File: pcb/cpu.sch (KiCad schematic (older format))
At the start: 8 parts, among them J100 Conn_02x05_Odd_Even, U100 LPC5500_FBD64

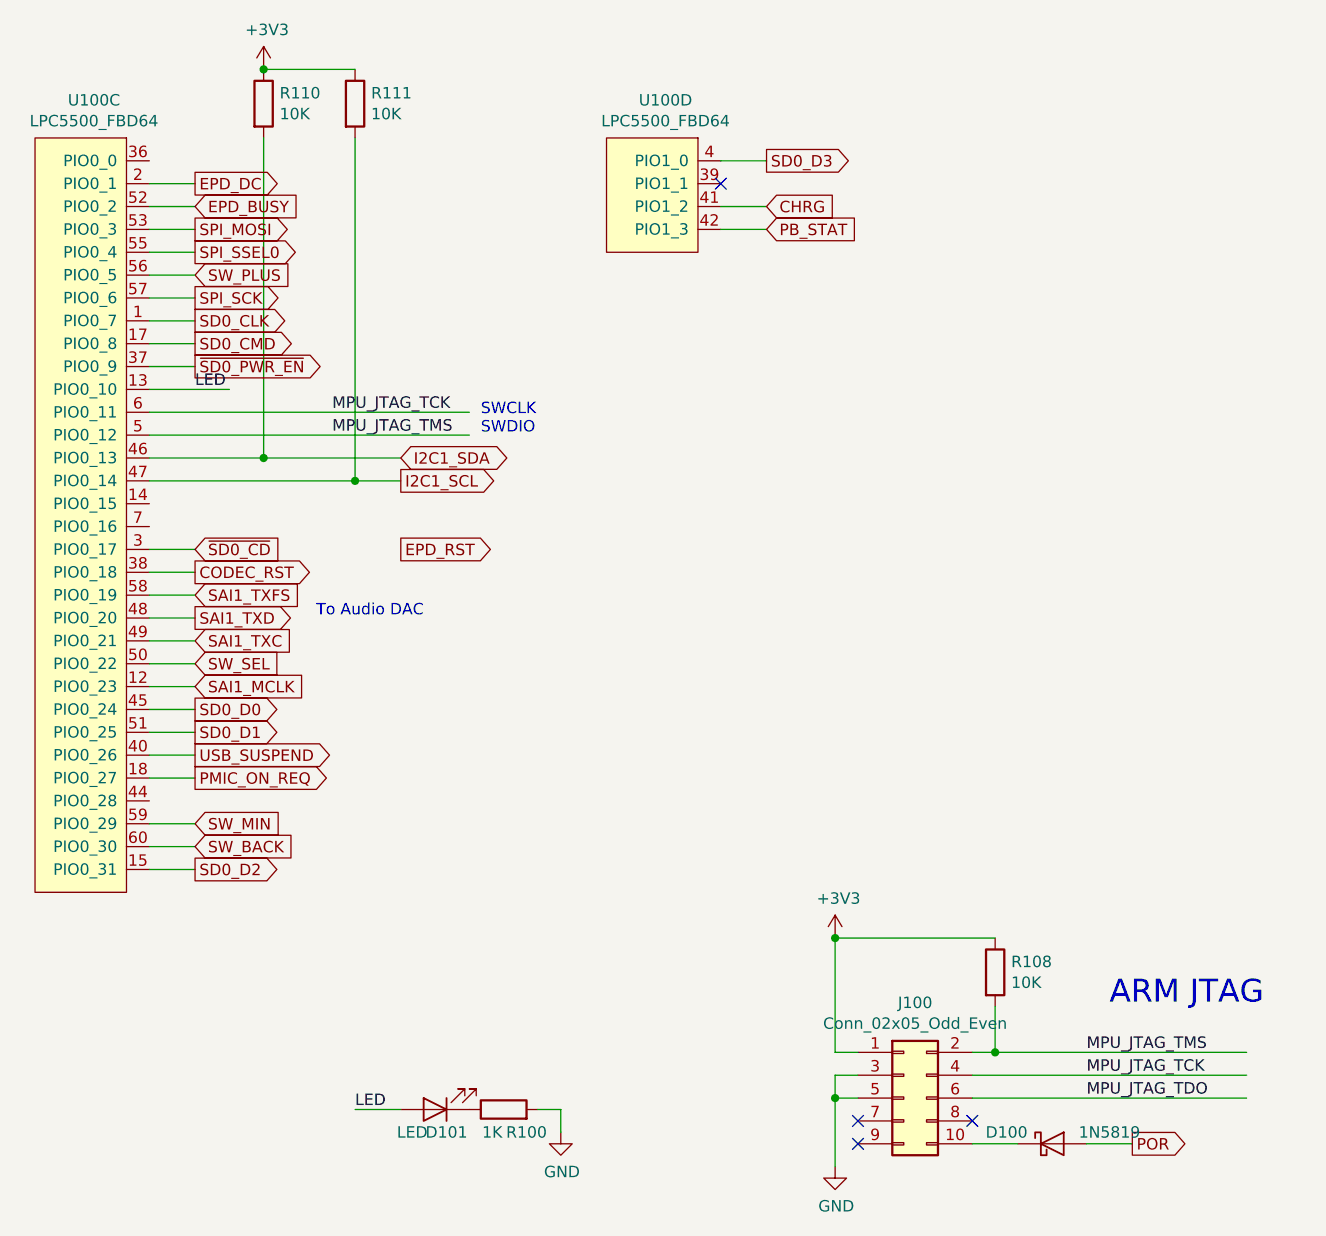
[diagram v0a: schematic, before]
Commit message: pcb: rev 0.2
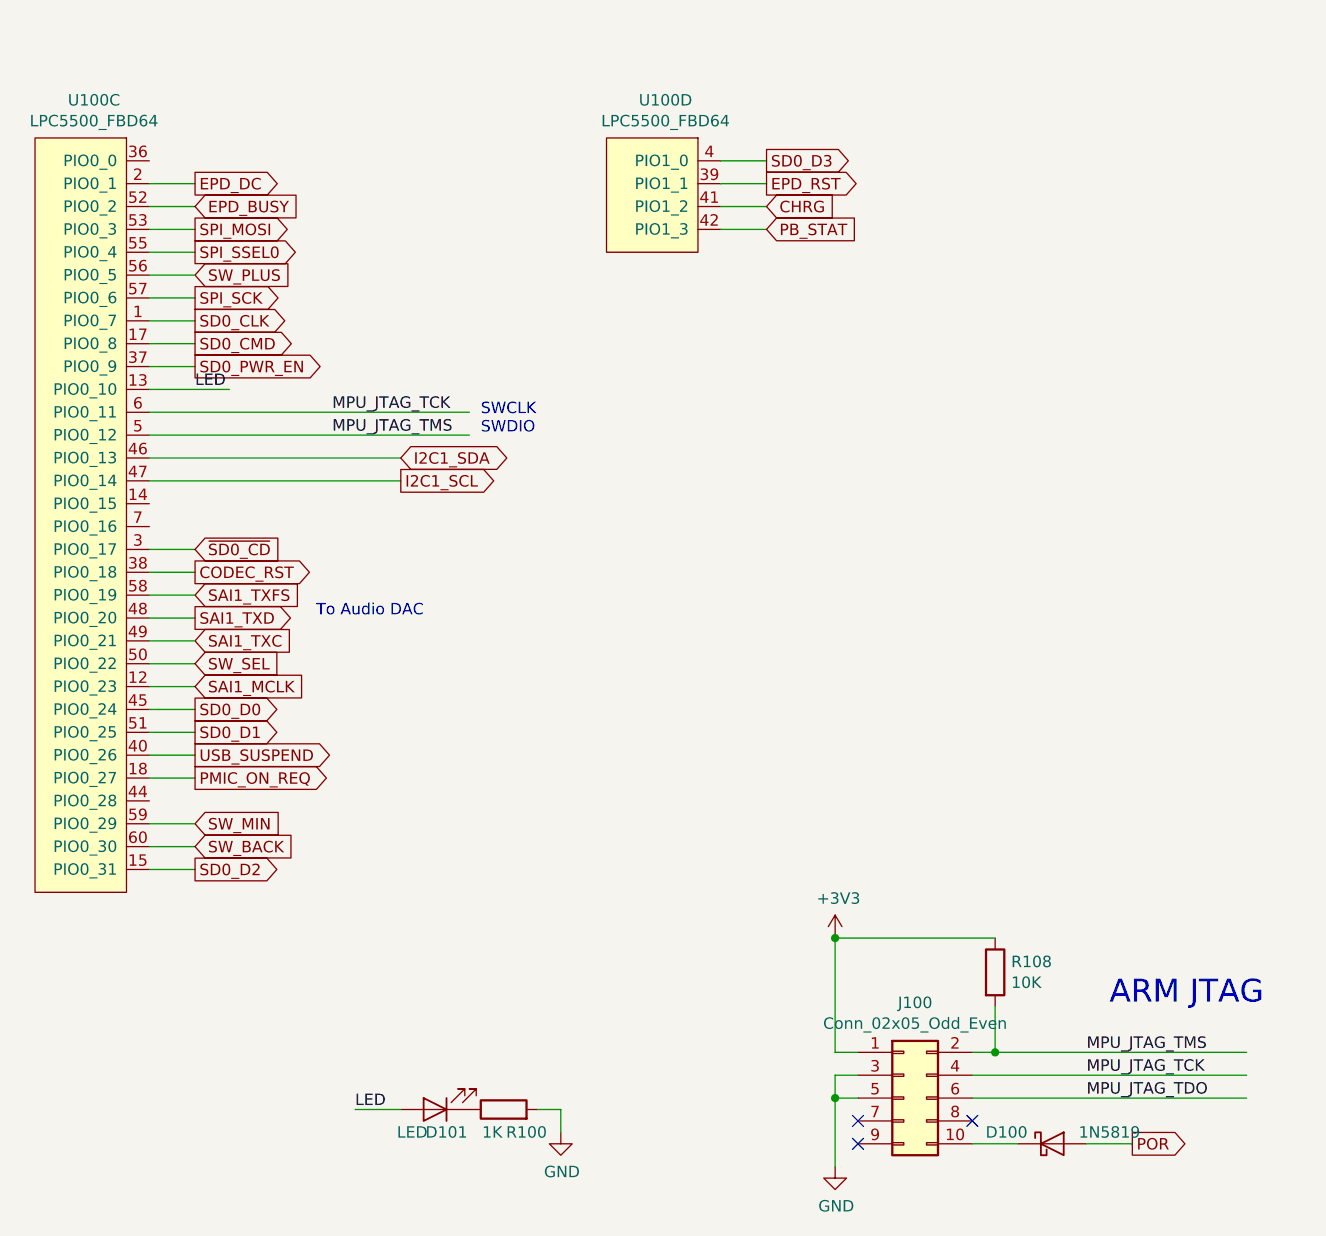
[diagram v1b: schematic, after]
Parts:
- removed R110, R111: 10K, Resistor_SMD:R_0603_1608Metric, symbol Device:R
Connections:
- net labels added: SD0_PWR_EN
- net labels removed: ~SD0_PWR_EN
- wire segments 53 -> 49
- no-connect marks 4 -> 3
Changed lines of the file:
@@
 To Audio DAC\n
 Text GLabel 4200 2700 2    50   Output ~ 0
-~SD0_PWR_EN
+SD0_PWR_EN
 Text GLabel 4200 2500 2    50   Output ~ 0
 SD0_CLK
@@
 Text GLabel 4200 3500 2    50   Input ~ 0
 ~SD0_CD
-Wire Wire Line
-	4900 1400 4500 1400
-$Comp
-L Device:R R111
-U 1 1 5DA7199D
-P 4900 1550
-F 0 "R111" H 4970 1596 50  0000 L CNN
-F 1 "10K" H 4970 1505 50  0000 L CNN
-F 2 "Resistor_SMD:R_0603_1608Metric" V 4830 1550 50  0001 C CNN
-F 3 "~" H 4900 1550 50  0001 C CNN
-	1    4900 1550
-	1    0    0    -1
-$EndComp
-$Comp
-L Device:R R110
-U 1 1 5DA710EB
-P 4500 1550
-F 0 "R110" H 4570 1596 50  0000 L CNN
-F 1 "10K" H 4570 1505 50  0000 L CNN
-F 2 "Resistor_SMD:R_0603_1608Metric" V 4430 1550 50  0001 C CNN
-F 3 "~" H 4500 1550 50  0001 C CNN
-	1    4500 1550
-	1    0    0    -1
-$EndComp
-Wire Wire Line
-	4000 3100 4500 3100
-Wire Wire Line
-	4500 1700 4500 3100
-Wire Wire Line
-	4900 1700 4900 3200
-Wire Wire Line
-	4000 3200 4900 3200
-Connection ~ 4900 3200
-Wire Wire Line
-	4900 3200 5100 3200
-Connection ~ 4500 3100
-Wire Wire Line
-	4500 3100 5100 3100
 Text GLabel 5100 3100 2    50   BiDi ~ 0
 I2C1_SDA
@@
 Wire Wire Line
 	4900 5950 5100 5950
-$Comp
-L power:+3V3 #PWR0106
-U 1 1 5DB9934B
-P 4500 1400
-F 0 "#PWR0106" H 4500 1250 50  0001 C CNN
-F 1 "+3V3" H 4515 1573 50  0000 C CNN
-F 2 "" H 4500 1400 50  0001 C CNN
-F 3 "" H 4500 1400 50  0001 C CNN
-	1    4500 1400
-	1    0    0    -1
-$EndComp
-Connection ~ 4500 1400
 Text GLabel 4200 3600 2    50   Output ~ 0
 CODEC_RST
@@
 Wire Wire Line
 	4000 1900 4200 1900
-NoConn ~ 6500 1900
 NoConn ~ 7600 6000
-Text GLabel 5100 3500 2    50   Output ~ 0
+Text GLabel 6700 1900 2    50   Output ~ 0
 EPD_RST
+Wire Wire Line
+	4000 3100 5100 3100
+Wire Wire Line
+	4000 3200 5100 3200
+Wire Wire Line
+	6500 1900 6700 1900
 $EndSCHEMATC
